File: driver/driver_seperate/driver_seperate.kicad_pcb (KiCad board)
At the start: 4 copper layers, 49.6 x 39.6 mm, 20 parts, among them IC1 MCT8316Z0TQRGFRQ1, J1 Conn_01x08_Pin, J2 Conn_01x05_Pin

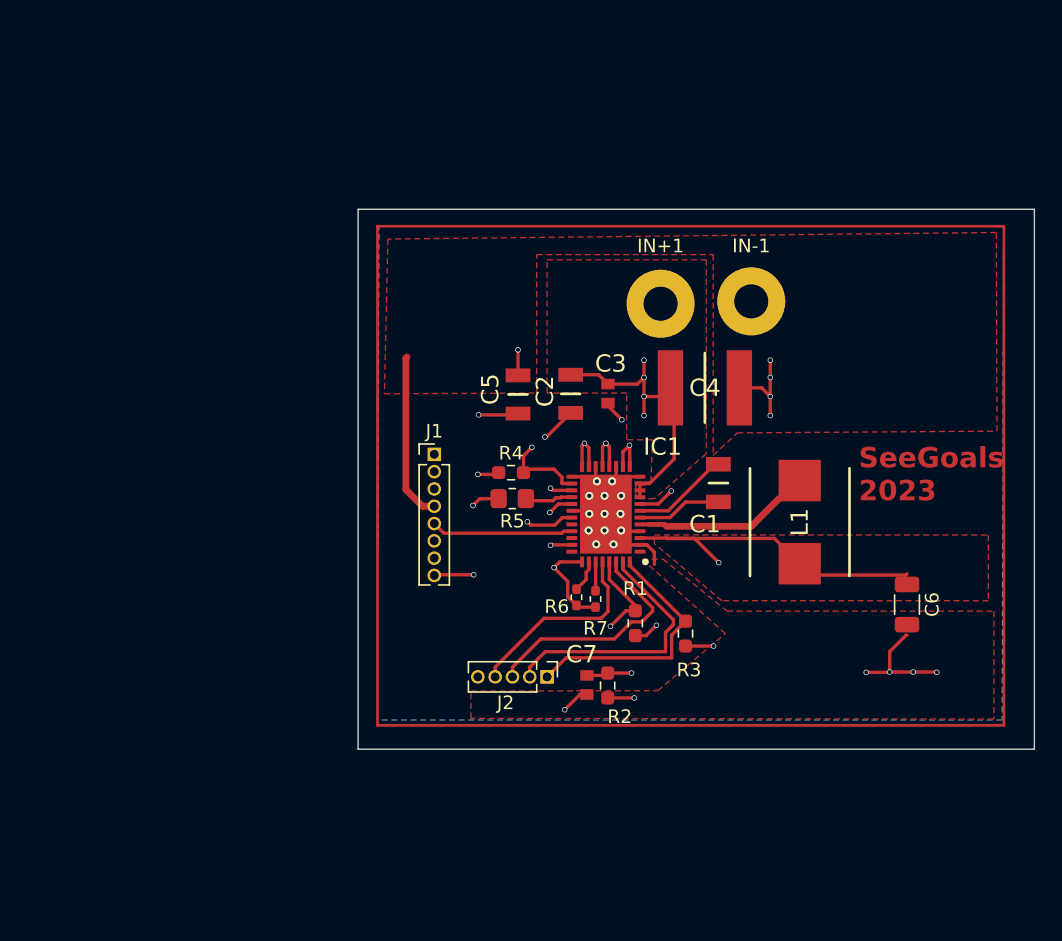
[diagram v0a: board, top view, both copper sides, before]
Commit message: Add newest version, revision started
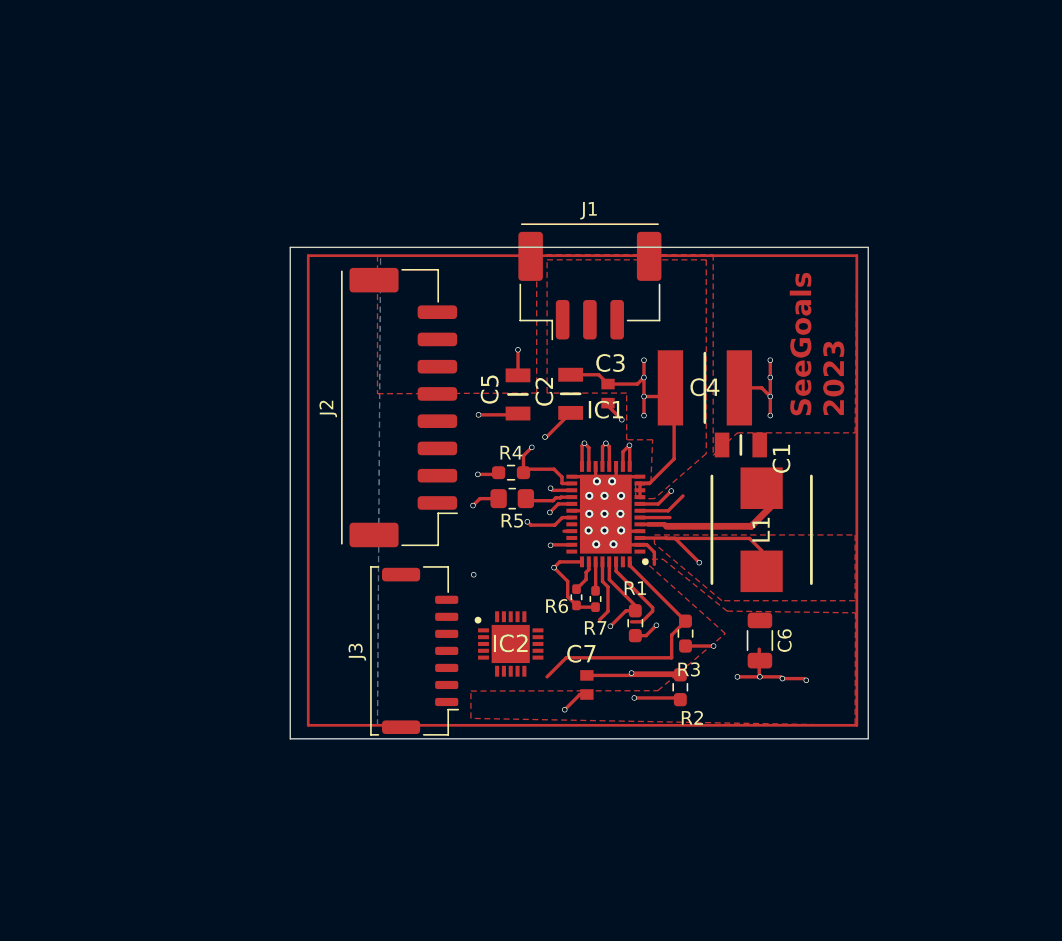
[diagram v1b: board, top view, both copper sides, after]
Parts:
- removed IN+1, IN-1: MountingHole_Pad, MountingHole:MountingHole_2.5mm_Pad
- added IC2: MCP23S08T-E_SO, SamacSys_Parts:QFN50P400X400X100-21N-D, F.Cu at (144.4, 109.2)
- added J3: Conn_01x07, Connector_Molex:Molex_CLIK-Mate_502382-0770_1x07-1MP_P1.25mm_Vertical, F.Cu at (137.8, 109.7)
- J1: value Conn_01x08_Pin -> Conn_01x03; footprint Connector_PinHeader_1.27mm:PinHeader_1x08_P1.27mm_Vertical -> Connector_Molex:Molex_CLIK-Mate_502443-0370_1x03-1MP_P2.00mm_Vertical
- J2: value Conn_01x05_Pin -> Motor; footprint Connector_PinHeader_1.27mm:PinHeader_1x05_P1.27mm_Vertical -> Connector_Molex:Molex_CLIK-Mate_502443-0870_1x08-1MP_P2.00mm_Vertical
- moved J2 22.4 mm to (136.5, 91.9), turned to 90 degrees
- moved J1 16.8 mm to (150.2, 82.9)
- moved C6 11.1 mm to (162.7, 109.0)
- moved R2 5.34 mm to (156.8, 112.4)
- moved C1 3.25 mm to (161.3, 94.6), turned to 0 degrees
- moved L1 2.85 mm to (162.8, 100.8)
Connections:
- IC1 pad 10: /VM -> /controller/VM
- IC1 pad 11: /VM -> /controller/VM
- IC1 pad 13: /U -> /controller/U
- IC1 pad 14: /U -> /controller/U
- IC1 pad 16: /V -> /controller/V
- IC1 pad 17: /V -> /controller/V
- IC1 pad 19: /W -> /controller/W
- IC1 pad 20: /W -> /controller/W
- IC1 pad 21: GND -> /controller/DRVOFF
- IC1 pad 22: /nFAULT -> /controller/nFAULT
- IC1 pad 23: /AVDD -> /controller/nSleep
- IC1 pad 25: /AVDD -> /controller/AVDD
- IC1 pad 27: /H1 -> /controller/H1
- IC1 pad 29: /H2 -> /controller/H2
- IC1 pad 3: /SW_BK -> /controller/SW_BK
- IC1 pad 31: /H3 -> /controller/H3
- IC1 pad 33: /AVDD -> /controller/AVDD
- IC1 pad 36: /DIR -> /controller/DIR
- IC1 pad 38: /BRAKE -> /controller/BRAKE
- IC1 pad 39: /PWM -> /controller/PWM
- IC1 pad 40: /FGOUT -> /controller/FGOUT
- IC1 pad 9: /VM -> /controller/VM
- J1 pad 1: /U -> /controller/VM
- J1 pad 2: /V -> /controller/+3V3
- J1 pad 3: /W -> GND
- J2 pad 1: /FGOUT -> /controller/U
- J2 pad 2: /PWM -> /controller/V
- J2 pad 3: /BRAKE -> /controller/W
- J2 pad 4: /DIR -> GND
- J2 pad 5: /nFAULT -> /controller/H2
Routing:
- net /nFAULT: track 34.7 -> 6.56 mm
- net /PWM: track 19.5 -> 0.00 mm
- net /U: track 19.4 -> 0.00 mm, vias 1 -> 0
- net /V: track 18.6 -> 0.00 mm, vias 1 -> 0
- net /BRAKE: track 17.4 -> 0.00 mm
- net /W: track 16.0 -> 0.00 mm, vias 1 -> 0
- net /SW_BK: track 46.9 -> 31.2 mm
- net /DIR: track 14.5 -> 0.00 mm
- net GND: track 48.6 -> 36.5 mm, vias 25 -> 24
- net /H1: track 11.3 -> 0.00 mm, vias 1 -> 0
- net /controller/U: track 0.00 -> 10.8 mm, vias 0 -> 1
- net /H3: track 10.5 -> 0.00 mm, vias 1 -> 0
- net /H2: track 10.5 -> 0.00 mm
- net Net-(IC1-ILIM): track 14.1 -> 21.3 mm
- net /controller/BRAKE: track 0.00 -> 6.60 mm
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- added copper zone on F.Cu, net /controller/VM
- added copper zone on In1.Cu, net /controller/VM
- removed copper zone on F.Cu, net /VM
- removed copper zone on In1.Cu, net /VM
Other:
- board size 49.6 x 39.6 mm -> 42.4 x 36.1 mm

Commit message: Add start of new design
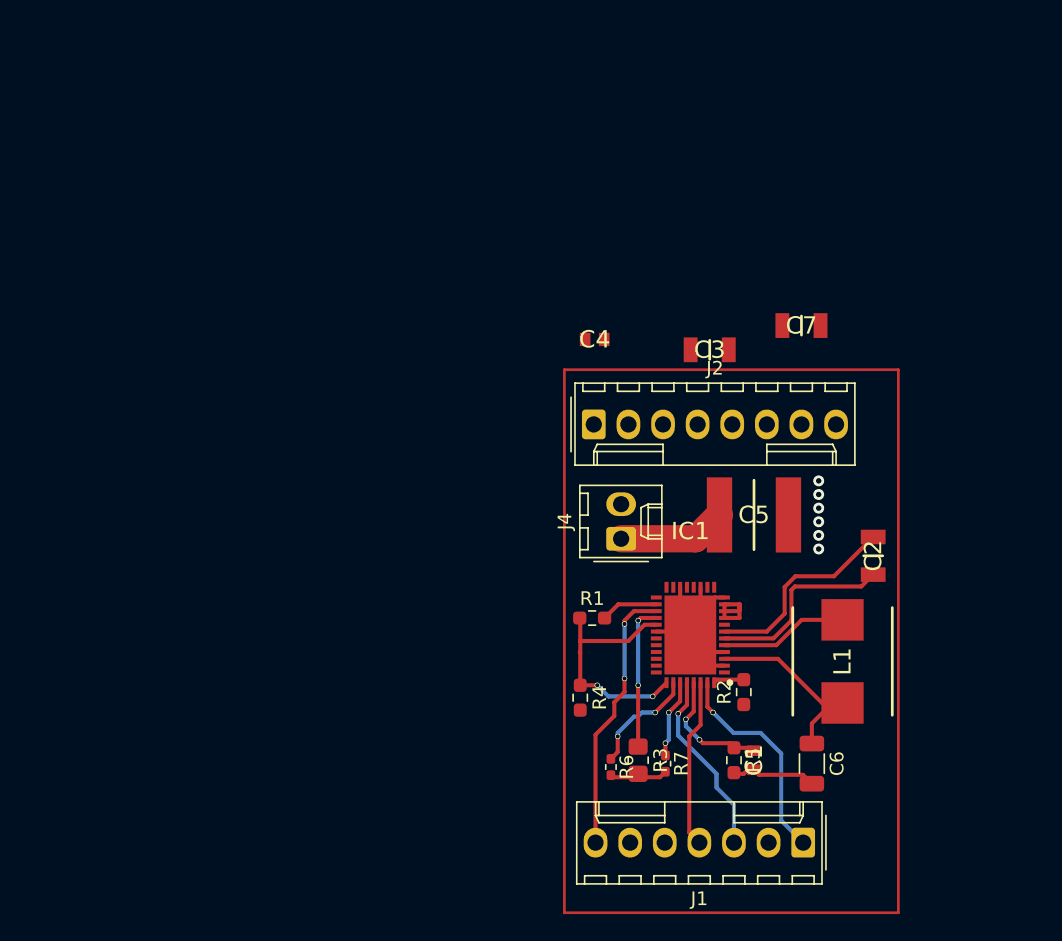
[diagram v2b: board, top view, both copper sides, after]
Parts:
- removed IC2: MCP23S08T-E_SO, SamacSys_Parts:QFN50P400X400X100-21N-D
- removed J3: Conn_01x07, Connector_Molex:Molex_CLIK-Mate_502382-0770_1x07-1MP_P1.25mm_Vertical
- added J4: Conn_01x02, Connector_Molex:Molex_KK-254_AE-6410-02A_1x02_P2.54mm_Vertical, F.Cu at (152.5, 101.5)
- C1: value 47nF -> 0u1F; footprint SamacSys_Parts:CAPC3216X180N -> SamacSys_Parts:CAPC1608X95N
- C2: value 1uF -> 47nF; footprint SamacSys_Parts:CAPC3216X178N -> SamacSys_Parts:CAPC3216X180N
- C3, C7: value 0u1F -> 1uF; footprint SamacSys_Parts:CAPC1608X95N -> SamacSys_Parts:CAPC3216X178N
- C4: value >=10uF -> 0u1F; footprint SamacSys_Parts:CAPC6153X500N -> SamacSys_Parts:CAPC1608X95N
- C5: value 1uF -> >=10uF; footprint SamacSys_Parts:CAPC3216X178N -> SamacSys_Parts:CAPC6153X500N
- J1: value Conn_01x03 -> Conn_01x07; footprint Connector_Molex:Molex_CLIK-Mate_502443-0370_1x03-1MP_P2.00mm_Vertical -> Connector_Molex:Molex_KK-254_AE-6410-07A_1x07_P2.54mm_Vertical
- J2: footprint Connector_Molex:Molex_CLIK-Mate_502443-0870_1x08-1MP_P2.00mm_Vertical -> Connector_Molex:Molex_KK-254_AE-6410-08A_1x08_P2.54mm_Vertical
- R1, R2: value 1k -> 5k1
- R3: value 5k1 -> 1M; footprint Resistor_SMD:R_0603_1608Metric_Pad0.98x0.95mm_HandSolder -> Resistor_SMD:R_0805_2012Metric_Pad1.20x1.40mm_HandSolder
- R4: value 5k1 -> 27k
- R5: value 1M -> 20k; footprint Resistor_SMD:R_0805_2012Metric_Pad1.20x1.40mm_HandSolder -> Resistor_SMD:R_0603_1608Metric_Pad0.98x0.95mm_HandSolder
- moved J1 43.8 mm to (165.9, 123.8), turned to 180 degrees
- moved C7 30.7 mm to (165.7, 85.9), turned to 0 degrees
- moved C2 25.2 mm to (171.0, 102.8), turned to -90 degrees
- moved R5 25.2 mm to (160.8, 117.8), turned to -90 degrees
- moved C1 23.2 mm to (162.2, 117.8), turned to -90 degrees
- moved C5 19.4 mm to (162.2, 99.8), turned to 0 degrees
- moved R4 17.3 mm to (149.5, 113.2), turned to -90 degrees
- moved J2 14.0 mm to (150.5, 93.1), turned to 0 degrees
- moved R7 13.1 mm to (155.8, 118.0)
- moved R6 12.7 mm to (151.8, 118.2)
- moved L1 11.3 mm to (168.8, 110.5)
- moved IC1 10.8 mm to (157.6, 108.6)
- moved R3 9.92 mm to (153.8, 117.8), turned to -90 degrees
- moved C6 9.81 mm to (166.5, 118.0)
- moved C4 8.84 mm to (150.6, 86.9)
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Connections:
- net /controller/H1 renamed /Motor Driver/H1
- net /controller/H2 renamed /Motor Driver/H2
- net /controller/H3 renamed /Motor Driver/H3
- net /controller/U renamed /Motor Driver/U
- net /controller/V renamed /Motor Driver/V
- net /controller/W renamed /Motor Driver/W
- C1 pad 1: Net-(IC1-CPH) -> Net-(IC1-ILIM)
- C1 pad 2: Net-(IC1-CPL) -> GND
- C2 pad 1: Net-(IC1-CP) -> Net-(IC1-CPH)
- C2 pad 2: /VM -> Net-(IC1-CPL)
- C3 pad 1: /VM -> Net-(IC1-CP)
- C3 pad 2: GND -> /Motor Driver/VM
- C4 pad 1: /VM -> /Motor Driver/VM
- C5 pad 1: /AVDD -> /Motor Driver/VM
- C6 pad 1: /SW_BK -> /Motor Driver/SW_BK
- C7 pad 1: Net-(IC1-ILIM) -> /Motor Driver/AVDD
- IC1 pad 10: /controller/VM -> /Motor Driver/VM
- IC1 pad 11: /controller/VM -> /Motor Driver/VM
- IC1 pad 21: /controller/DRVOFF -> /Motor Driver/DRVOFF
- IC1 pad 22: /controller/nFAULT -> /Motor Driver/nFAULT
- IC1 pad 23: /controller/nSleep -> /Motor Driver/nSleep
- IC1 pad 25: /controller/AVDD -> /Motor Driver/AVDD
- IC1 pad 3: /controller/SW_BK -> /Motor Driver/SW_BK
- IC1 pad 33: /controller/AVDD -> /Motor Driver/AVDD
- IC1 pad 36: /controller/DIR -> /Motor Driver/DIR
- IC1 pad 38: /controller/BRAKE -> /Motor Driver/BRAKE
- IC1 pad 39: /controller/PWM -> /Motor Driver/PWM
- IC1 pad 40: /controller/FGOUT -> /Motor Driver/FGOUT
- IC1 pad 9: /controller/VM -> /Motor Driver/VM
- J1 pad 1: /controller/VM -> /Motor Driver/PWM
- J1 pad 2: /controller/+3V3 -> /Motor Driver/FGOUT
- J1 pad 3: GND -> /Motor Driver/DIR
- J2 pad 8: /controller/SW_BK -> /Motor Driver/SW_BK
- L1 pad 2: /SW_BK -> /Motor Driver/SW_BK
- R1 pad 1: /AVDD -> /Motor Driver/AVDD
- R1 pad 2: Net-(IC1-ILIM) -> /Motor Driver/nFAULT
- R2 pad 1: Net-(IC1-ILIM) -> /Motor Driver/AVDD
- R2 pad 2: GND -> /Motor Driver/FGOUT
- R3 pad 1: /AVDD -> Net-(IC1-VSEL_BK)
- R3 pad 2: /FGOUT -> /Motor Driver/AVDD
- R4 pad 1: /AVDD -> /Motor Driver/AVDD
- R4 pad 2: /nFAULT -> Net-(IC1-ILIM)
- R5 pad 1: Net-(IC1-VSEL_BK) -> Net-(IC1-ILIM)
- R5 pad 2: /AVDD -> GND
- R6 pad 2: /AVDD -> /Motor Driver/AVDD
- R7 pad 2: /AVDD -> /Motor Driver/AVDD
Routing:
- net /SW_BK: track 31.2 -> 0.00 mm, vias 2 -> 0
- net /Motor Driver/AVDD: track 0.00 -> 22.6 mm, vias 0 -> 2
- net /VM: track 21.9 -> 0.00 mm, vias 3 -> 0
- net /Motor Driver/nSleep: track 0.00 -> 19.8 mm, vias 0 -> 2
- net /FGOUT: track 18.9 -> 0.00 mm
- net /AVDD: track 17.7 -> 0.00 mm, vias 6 -> 0
- net Net-(IC1-CP): track 17.1 -> 0.00 mm, vias 2 -> 0
- net /Motor Driver/PWM: track 0.00 -> 15.8 mm, vias 0 -> 1
- net /Motor Driver/SW_BK: track 0.00 -> 14.4 mm
- net /Motor Driver/VM: track 0.00 -> 13.7 mm
- net /Motor Driver/DIR: track 0.00 -> 13.7 mm, vias 0 -> 1
- net /Motor Driver/BRAKE: track 0.00 -> 12.4 mm
- net Net-(IC1-ILIM): track 21.3 -> 9.18 mm
- net Net-(IC1-CPL): track 2.20 -> 14.2 mm
- net Net-(IC1-CPH): track 3.61 -> 14.9 mm
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- added copper zone on In2.Cu, net /Motor Driver/VM
- added copper zone on In1.Cu, net GND
- removed copper zone on In2.Cu, net /AVDD
- removed copper zone on F.Cu, net /SW_BK
- removed copper zone on F.Cu, net /controller/VM
- removed copper zone on In1.Cu, net /controller/VM
- removed copper zone on B.Cu, net GND
- removed copper zone on F.Cu, net GND
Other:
- board outline removed
- board text removed: "SeeGoals 2023"

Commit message: Add new design
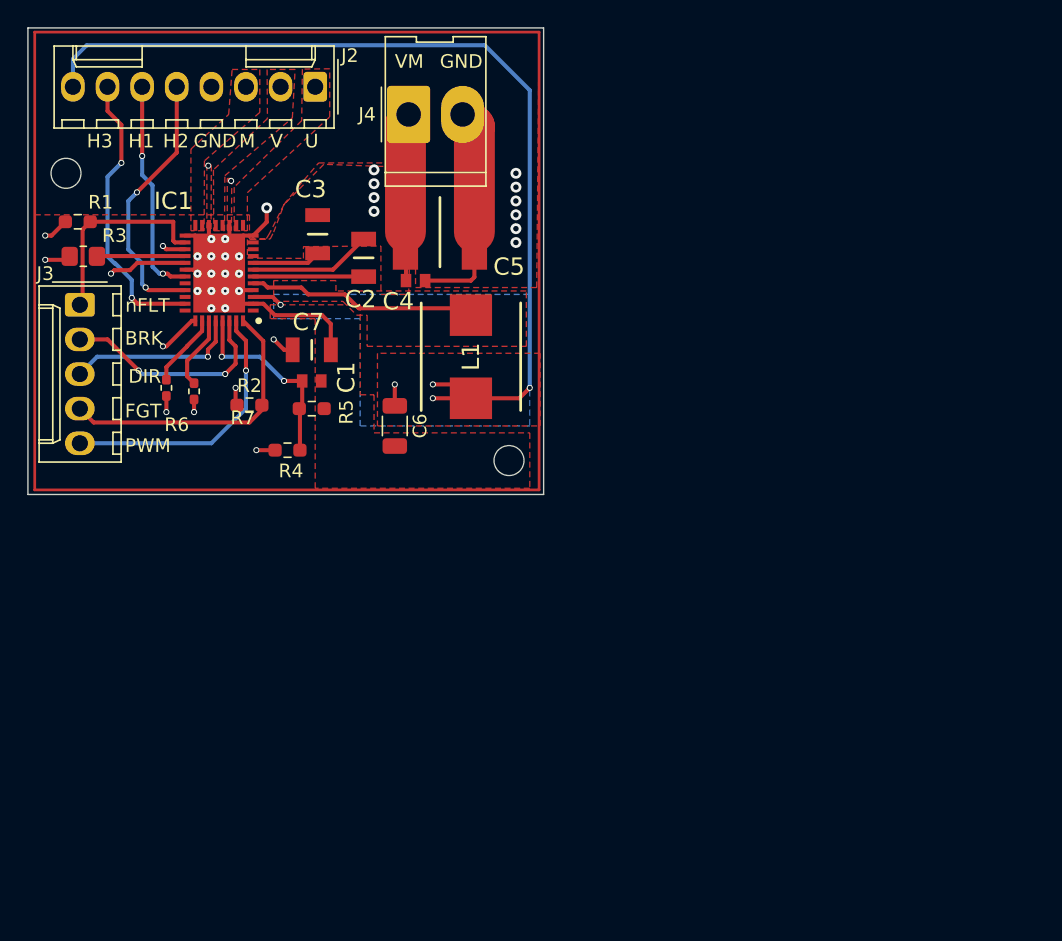
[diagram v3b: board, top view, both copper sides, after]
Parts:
- removed J1: Conn_01x07, Connector_Molex:Molex_KK-254_AE-6410-07A_1x07_P2.54mm_Vertical
- added H1: MountingHole, MountingHole:MountingHole_2.2mm_M2, F.Cu at (144.3, 95.8)
- added H2: MountingHole, MountingHole:MountingHole_2.2mm_M2, F.Cu at (111.8, 74.7)
- added J3: Conn_01x05, Connector_Molex:Molex_KK-254_AE-6410-05A_1x05_P2.54mm_Vertical, F.Cu at (112.8, 84.3)
- J4: footprint Connector_Molex:Molex_KK-254_AE-6410-02A_1x02_P2.54mm_Vertical -> Connector_Molex:Molex_KK-396_5273-02A_1x02_P3.96mm_Vertical
- moved R3 55.0 mm to (113.0, 80.8), turned to 180 degrees
- moved R1 47.7 mm to (112.6, 78.2)
- moved R7 44.1 mm to (121.2, 90.7)
- moved IC1 43.6 mm to (123.0, 82.0)
- moved C2 43.3 mm to (133.6, 80.9)
- moved R6 42.9 mm to (119.1, 90.4)
- moved C1 42.8 mm to (129.8, 89.9), turned to 0 degrees
- moved R2 41.9 mm to (125.2, 91.7), turned to 0 degrees
- moved R5 40.3 mm to (129.8, 91.9), turned to 0 degrees
- moved C6 39.4 mm to (135.9, 93.2)
- moved C7 36.0 mm to (129.8, 87.6)
- moved L1 35.3 mm to (141.5, 88.1)
- moved J4 34.8 mm to (136.9, 70.4), turned to 0 degrees
- moved J2 32.1 mm to (130.0, 68.3), turned to 180 degrees
- moved C5 31.0 mm to (139.2, 79.0)
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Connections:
- net /Motor Driver/nFAULT renamed /Motor Driver/nFault
- IC1 pad 21: /Motor Driver/DRVOFF -> GND
- IC1 pad 23: /Motor Driver/nSleep -> /Motor Driver/AVDD
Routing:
- net /Motor Driver/SW_BK: track 14.4 -> 73.7 mm, vias 0 -> 5
- net GND: track 27.5 -> 52.7 mm, vias 6 -> 25
- net /Motor Driver/H3: track 0.00 -> 21.2 mm, vias 0 -> 2
- net /Motor Driver/nSleep: track 19.8 -> 0.00 mm, vias 2 -> 0
- net /Motor Driver/H2: track 0.00 -> 19.7 mm, vias 0 -> 2
- net /Motor Driver/FGOUT: track 2.26 -> 21.4 mm
- net /Motor Driver/H1: track 0.00 -> 16.2 mm, vias 0 -> 2
- net /Motor Driver/nFault: track 4.21 -> 14.8 mm
- net Net-(IC1-SW_BK): track 9.44 -> 16.9 mm
- net Net-(IC1-CPL): track 14.2 -> 8.11 mm
- net Net-(IC1-CPH): track 14.9 -> 9.04 mm
- net Net-(IC1-ILIM): track 9.18 -> 14.5 mm
- net /Motor Driver/VM: track 13.7 -> 18.8 mm, vias 0 -> 4
- net Net-(IC1-CP): track 0.00 -> 5.02 mm
- net Net-(IC1-VSEL_BK): track 10.7 -> 6.48 mm, vias 2 -> 0
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- added copper zone on In2.Cu, net /Motor Driver/AVDD
- added copper zone on B.Cu, net /Motor Driver/SW_BK
- added copper zone on F.Cu, net /Motor Driver/SW_BK
- added copper zone on F.Cu, net /Motor Driver/U
- added copper zone on F.Cu, net /Motor Driver/V
- added copper zone on F.Cu, net /Motor Driver/VM
- added copper zone on F.Cu, net /Motor Driver/W
- added copper zone on F.Cu, net GND
- added copper zone on F.Cu, net Net-(IC1-SW_BK)
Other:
- board outline added: 37.8 x 34.2 mm
- board text added: "BRK"
- board text added: "DIR"
- board text added: "FGT"
- board text added: "GND"
- board text added: "H1"
- board text added: "H2"
- board text added: "H3"
- board text added: "M"
- board text added: "PWM"
- board text added: "SeeGoals 2024 Motor driver v2"
- board text added: "U"
- board text added: "V"
- board text added: "VM"
- board text added: "nFLT"
